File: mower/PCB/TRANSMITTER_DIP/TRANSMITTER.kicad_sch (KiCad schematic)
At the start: 16 parts, among them J1 BOT POWER, J2 POWER IN, J3 SHUNT, J4 COIL OUT, J5 COIL POWER IN, Q1 IRF3205, U1 LM358, U4 LM555xN

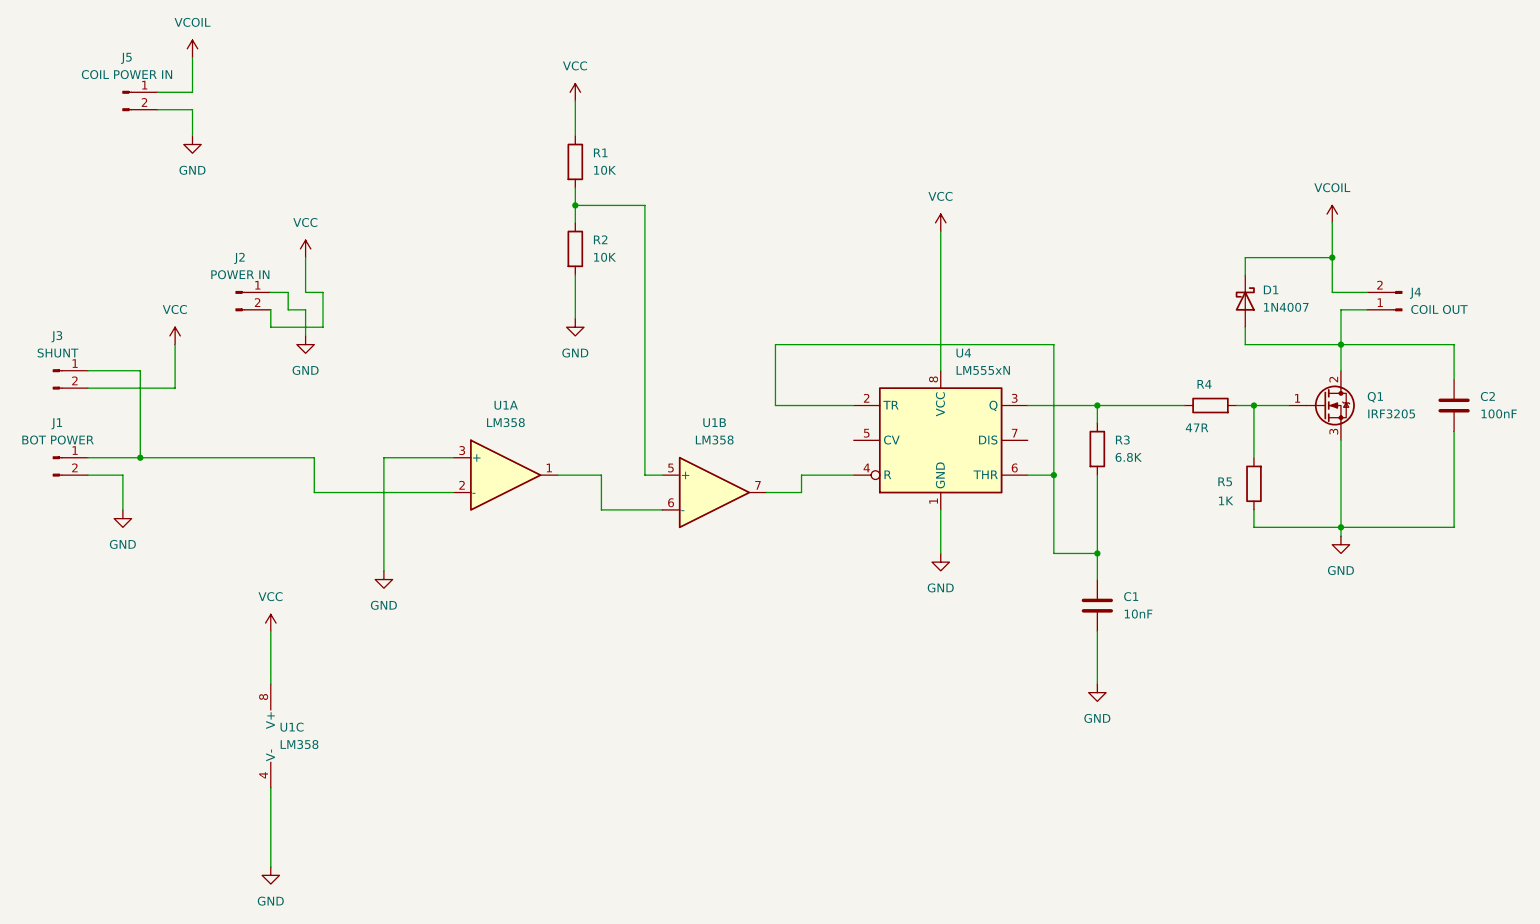
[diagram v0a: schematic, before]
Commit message: Consolidate complete mower design (all branches) + zana repo structure
Mower fragments from every botkorp branch (mowbot3/4, TRANSMITTER_SMD,
IMRANS_LIBRARY) unioned into mower/. Adds legacy/opengro, README, .gitignore.
Sits on top of the preserved 13-commit mower history.

Co-Authored-By: Claude Opus 4.8 <noreply@anthropic.com>
Claude-Session: https://claude.ai/code/session_017QXBEryTihUadNUZqQzfmo
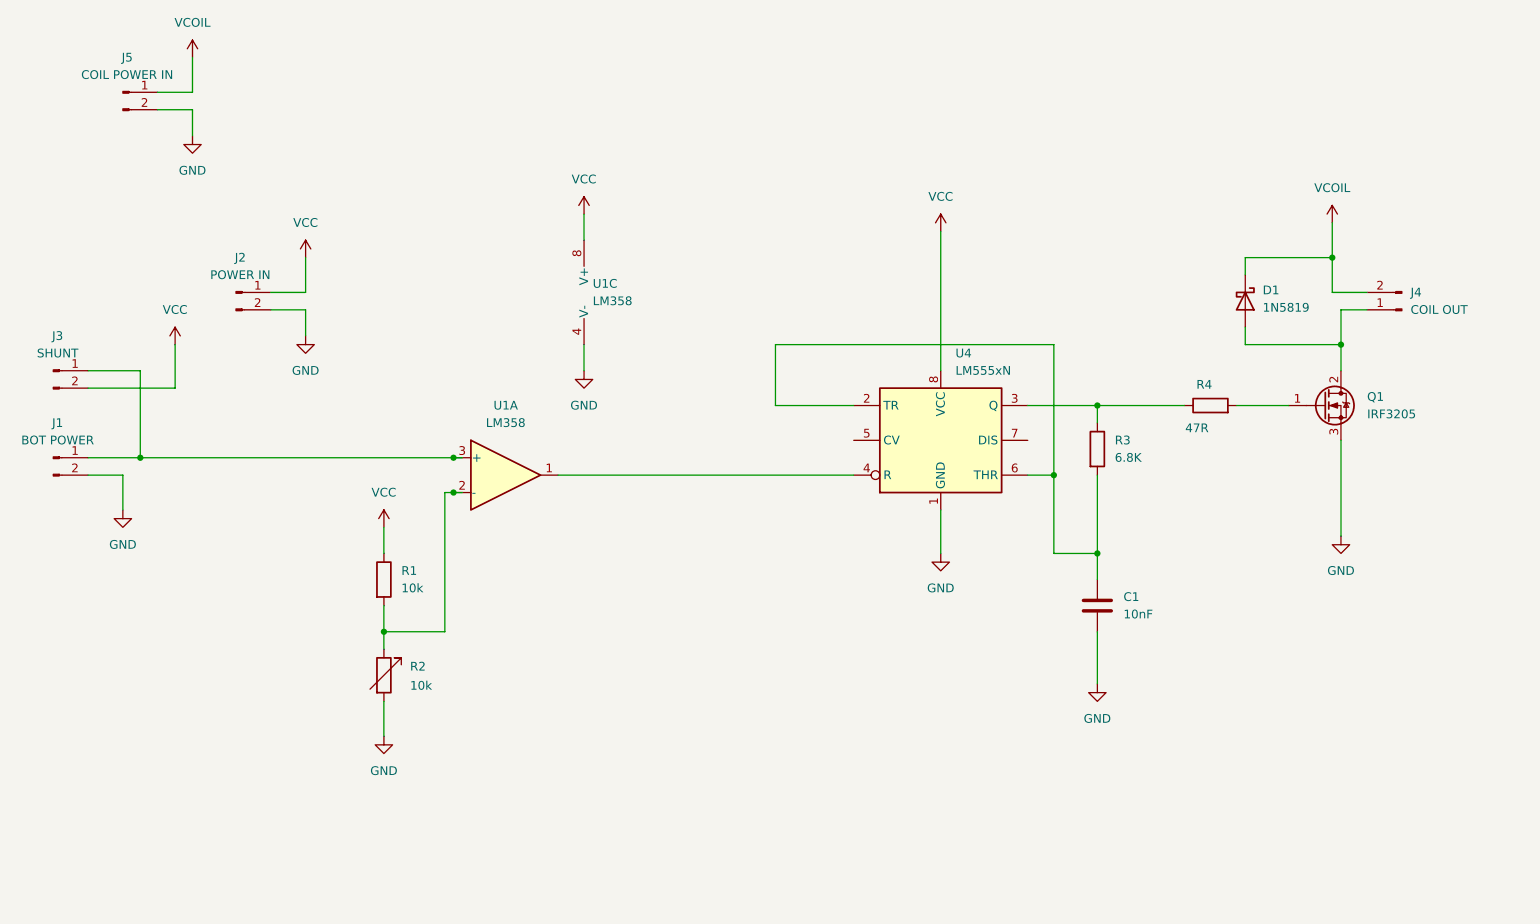
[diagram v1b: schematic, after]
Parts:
- removed C2: 100nF, IMRANS_LIBRARY:C_Disc_D3.0mm_W1.6mm_P2.50mm, symbol Device:C
- removed R2: 10K, IMRANS_LIBRARY:R_Axial_DIN0207_L6.3mm_D2.5mm_P10.16mm_Horizontal_2, symbol Device:R
- removed R5: 1K, IMRANS_LIBRARY:R_Axial_DIN0207_L6.3mm_D2.5mm_P10.16mm_Horizontal_2, symbol Device:R
- removed unit 2 of U1
- added R2: 10k, IMRANS_LIBRARY:Potentiometer_Bourns_3386P_Vertical, symbol Device:R_Variable
- D1: value 1N4007 -> 1N5819
- R1: value 10K -> 10k
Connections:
- net GND: now also J2.2 (Pin_2), R2.2; no longer J2.1 (Pin_1), U1.3 (+)
- net VCC: now also J2.1 (Pin_1); no longer J2.2 (Pin_2)
- net at U4.4 (R): now also U1.1
- net at J1.1 (Pin_1), J3.1 (Pin_1): now also U1.3 (+); no longer U1.2 (-)
- net at R1.2: now also U1.2 (-), R2.1
